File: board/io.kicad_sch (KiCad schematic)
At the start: 32 parts, among them J2 KEYBOARD, J4 MOUSE, J5 AudioJack2, J9 FTDI serial, U15 LM358, U16 AT89x51xxP, Y2 11.0592MHz

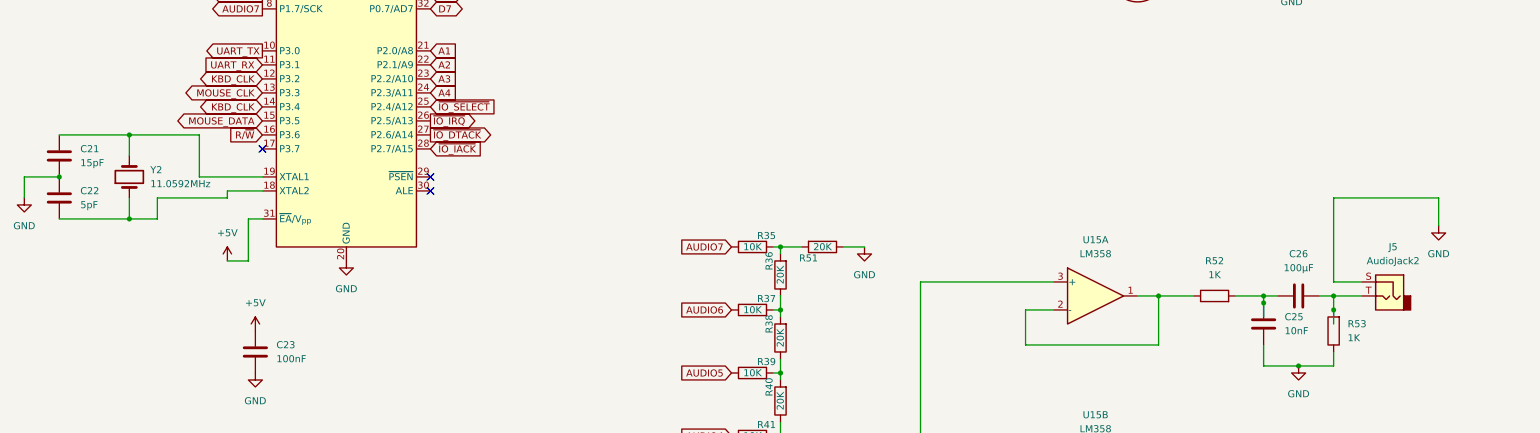
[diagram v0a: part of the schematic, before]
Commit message: design draft complete, added footprints
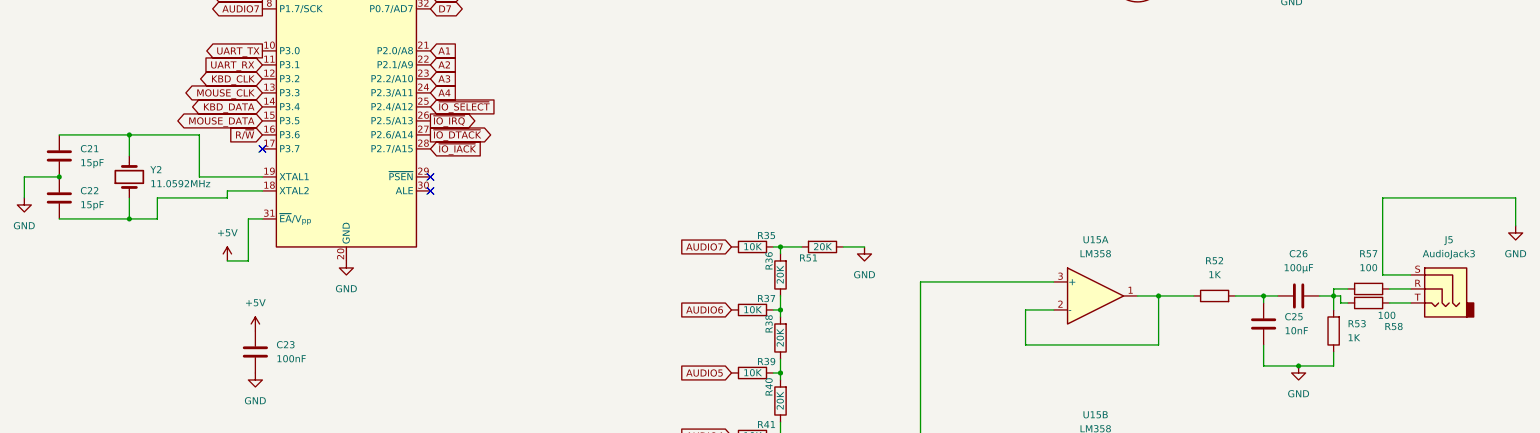
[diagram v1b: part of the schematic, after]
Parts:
- removed J5: AudioJack2, symbol Connector_Audio:AudioJack2
- added J5: AudioJack3, Connector_Audio:Jack_3.5mm_CUI_SJ1-3523N_Horizontal, symbol Connector_Audio:AudioJack3
- added R57, R58: 100, Resistor_THT:R_Axial_DIN0207_L6.3mm_D2.5mm_P10.16mm_Horizontal, symbol Device:R
- C21, C25: footprint (none) -> Capacitor_THT:C_Disc_D3.0mm_W1.6mm_P2.50mm
- C22: value 5pF -> 15pF; footprint (none) -> Capacitor_THT:C_Disc_D3.0mm_W1.6mm_P2.50mm
- C23, C24: footprint (none) -> Capacitor_THT:C_Disc_D5.0mm_W2.5mm_P5.00mm
- C26: footprint (none) -> Capacitor_THT:CP_Radial_D5.0mm_P2.50mm
- J2, J4: footprint (none) -> board:Mini_din6
- J9: footprint (none) -> Connector_PinHeader_2.54mm:PinHeader_1x06_P2.54mm_Vertical
- R35, R36, R37, R38, R39, R40, R41, R42, R43, R44, R45, R46, R47, R48, R49, R50, R51, R52, R53: footprint (none) -> Resistor_THT:R_Axial_DIN0207_L6.3mm_D2.5mm_P10.16mm_Horizontal
- U15: footprint (none) -> Package_DIP:DIP-8_W7.62mm
- Y2: footprint (none) -> Crystal:Resonator-2Pin_W10.0mm_H5.0mm
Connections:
- net GND: now also J5.S
- net KBD_CLK: no longer U16.14 (P3.4)
- net KBD_DATA: now also U16.14 (P3.4)
- net at C26.2, R53.2: now also R57.2, R58.2
- new net: J5.R, R57.1
- new net: J5.T, R58.1
